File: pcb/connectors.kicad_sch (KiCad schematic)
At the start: 3 parts, among them J20 DTM1312PA12PBR008, U8 EEC-325X4B

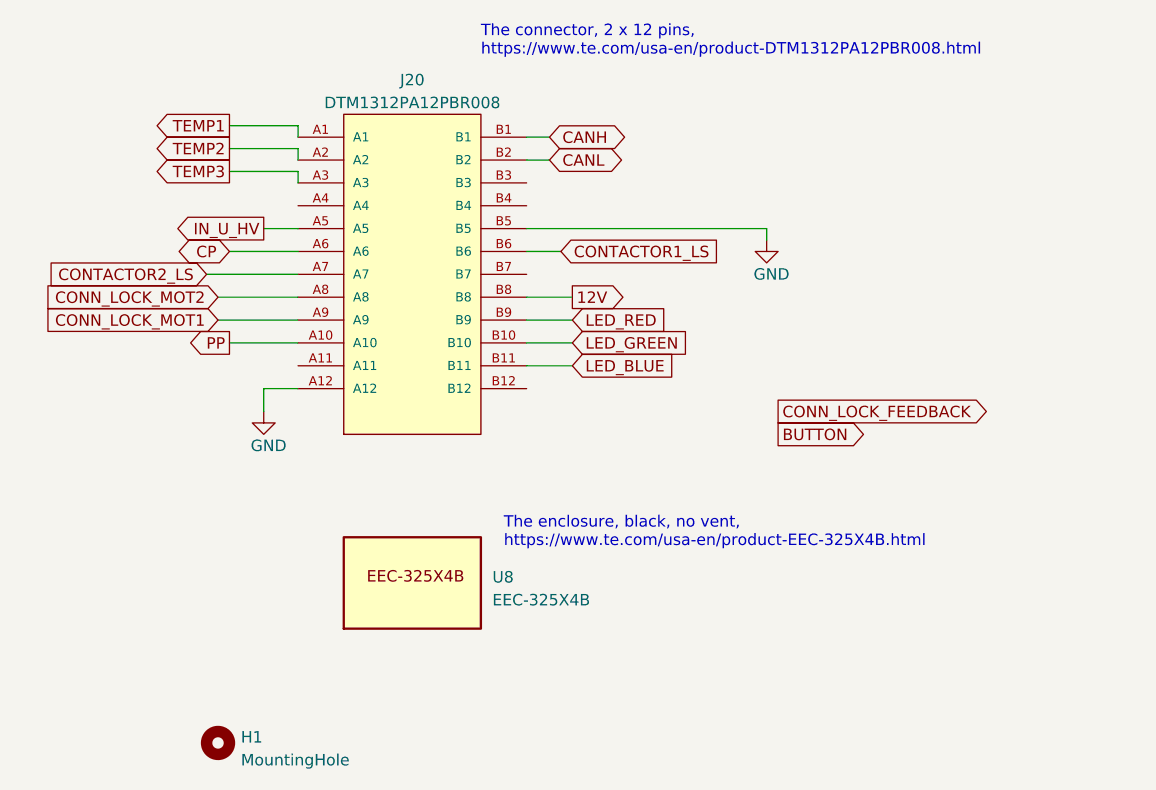
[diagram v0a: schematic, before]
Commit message: wired the drv8874. Added spare holes. Flash connector larger holes
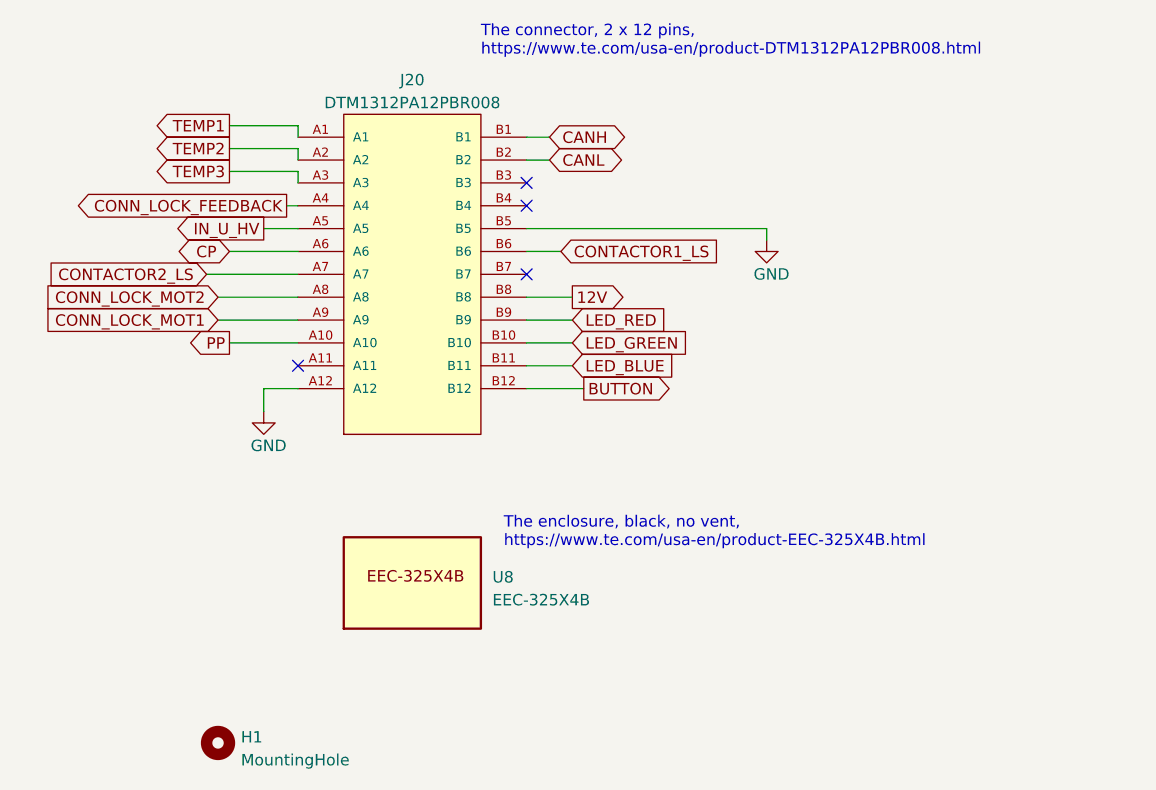
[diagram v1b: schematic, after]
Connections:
- net BUTTON: now also J20.B12
- net CONN_LOCK_FEEDBACK: now also J20.A4
- no-connect marks 0 -> 4
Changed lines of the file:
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@@
 (kicad_sch (version 20230121) (generator eeschema)
   (paper "A4")
+  (no_connect (at 78.74 49.53))
+  (no_connect (at 78.74 59.69))
+  (no_connect (at 78.74 52.07))
+  (no_connect (at 53.34 69.85))
+  (wire (pts (xy 52.07 52.07) (xy 53.34 52.07))
+    (stroke (width 0) (type default))
+  )
   (wire (pts (xy 53.34 43.18) (xy 53.34 44.45))
+    (stroke (width 0) (type default))
+  )
+  (wire (pts (xy 78.74 72.39) (xy 85.09 72.39))
     (stroke (width 0) (type default))
   )
@@
     )
   )
-  (global_label "BUTTON" (shape output) (at 106.68 77.47 0) (fields_autoplaced)
+  (global_label "BUTTON" (shape output) (at 85.09 72.39 0) (fields_autoplaced)
     (effects (font (size 1.27 1.27)) (justify left))
-    (property "Intersheetrefs" "${INTERSHEET_REFS}" (at 116.7825 77.47 0)
+    (property "Intersheetrefs" "${INTERSHEET_REFS}" (at 95.1925 72.39 0)
       (effects (font (size 1.27 1.27)) (justify left) hide)
     )
@@
     )
   )
-  (global_label "CONN_LOCK_FEEDBACK" (shape output) (at 106.68 74.93 0) (fields_autoplaced)
-    (effects (font (size 1.27 1.27)) (justify left))
-    (property "Intersheetrefs" "${INTERSHEET_REFS}" (at 131.2363 74.93 0)
-      (effects (font (size 1.27 1.27)) (justify left) hide)
+  (global_label "CONN_LOCK_FEEDBACK" (shape output) (at 52.07 52.07 180) (fields_autoplaced)
+    (effects (font (size 1.27 1.27)) (justify right))
+    (property "Intersheetrefs" "${INTERSHEET_REFS}" (at 27.5137 52.07 0)
+      (effects (font (size 1.27 1.27)) (justify right) hide)
     )
   )

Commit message: changed to 4 layers. Added button, PP and lock feedback. New testpoints to avoid courtyard warnings.
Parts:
- J20: footprint TE_DTM1312PA12PBR008 -> DTM1312PA12PBR008:TE_DTM1312PA12PBR008
- U8: footprint TE_EEC-325X4B -> EEC-325X4B:TE_EEC-325X4B
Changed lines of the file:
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@@
       (effects (font (size 1.27 1.27)))
     )
-    (property "Footprint" "TE_DTM1312PA12PBR008" (at 66.04 57.15 0)
+    (property "Footprint" "DTM1312PA12PBR008:TE_DTM1312PA12PBR008" (at 66.04 57.15 0)
       (effects (font (size 1.27 1.27)) (justify left bottom) hide)
     )
@@
       (effects (font (size 1.27 1.27)) (justify left))
     )
-    (property "Footprint" "TE_EEC-325X4B" (at 63.5 93.98 0)
+    (property "Footprint" "EEC-325X4B:TE_EEC-325X4B" (at 63.5 93.98 0)
       (effects (font (size 1.27 1.27)) (justify left bottom) hide)
     )
